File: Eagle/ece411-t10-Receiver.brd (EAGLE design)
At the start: 9.3 x 17.3 mm, 10 parts, among them X1 22-23-2021, X2 22-23-2021

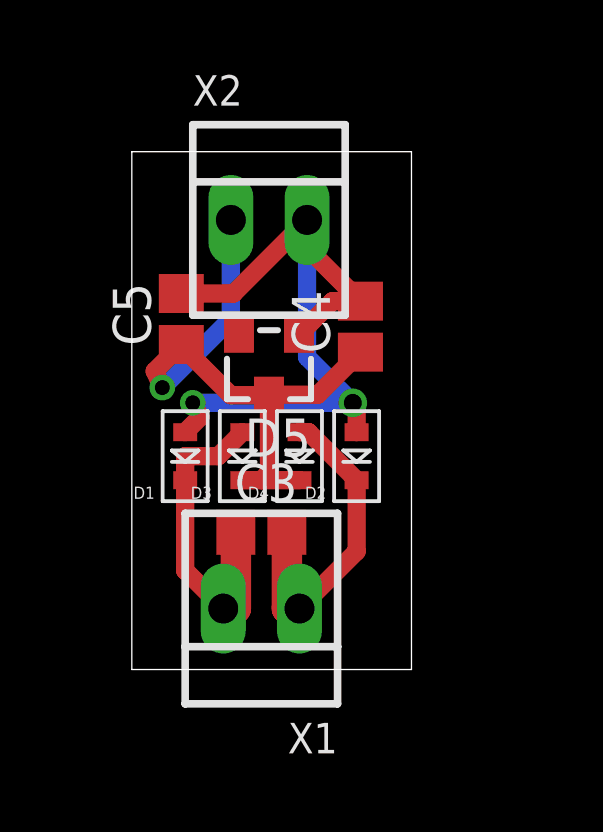
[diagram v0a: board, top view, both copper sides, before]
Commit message: Boards + schematics rev2
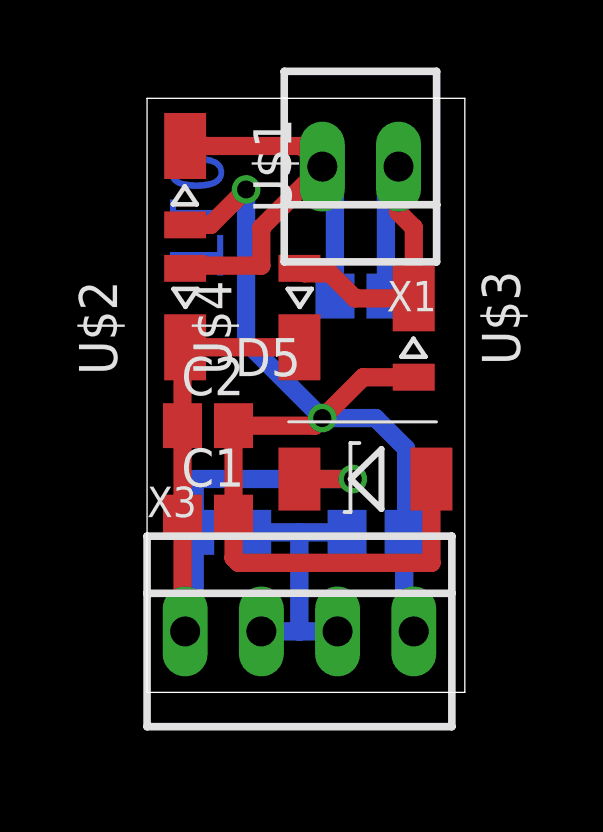
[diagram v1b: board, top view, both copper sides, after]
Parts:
- removed C4, C5: (no value), adafruit:C0805
- removed D1, D2, D3, D4: DFLS230LQ-7, adafruit:SOD-523
- removed X2: 22-23-2021, con-molex:22-23-2021
- added C1: 100n+, adafruit:C0805
- added C2: 100n, adafruit:C0805
- added R1: 75k, resistor:R0805
- added R2: 51k, resistor:R0805
- added U$1, U$2, U$3, U$4: DFLS230LQ-SCHOTTKY, _VMS:PWRDI123
- added X3: USB, con-molex:22-23-2041
- C3: value (none) -> NP
- D5: value 5.1V -> DZ2405100LCT-ZENER; device diode:TO236 -> _VMS:ZENER_PWR_PKG
- moved X1 15.1 mm to (7.11, 17.3)
- moved C3 8.54 mm to (7.11, 13.0), flipped to the bottom, turned to 180 degrees
- moved D5 3.94 mm to (5.08, 6.86), turned to 0 degrees
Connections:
- removed net N$3: C4.2, C5.2, D1.A, D2.A, D5.A, X2.2
- new net N$5: R1.1, R2.2, X3.2, X3.3
- new net N$8: C1.2, C2.2, D5.A, R2.1, U$1.A, U$3.A, X3.4
- net N$1: now also U$1.C, U$2.A; no longer D1.K, D3.A
- net N$2: now also U$3.C, U$4.A; no longer D2.K, D4.A
- net N$4: now also C1.1, C2.1, R1.2, U$2.C, U$4.C, X3.1; no longer C4.1, C5.1, D3.K, D4.K, X2.1
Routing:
- net N$8: track 0.00 -> 41.2 mm, vias 0 -> 2
- net N$3: track 25.5 -> 0.00 mm, vias 2 -> 0
- net N$5: track 0.00 -> 9.02 mm
- net N$1: track 10.8 -> 16.1 mm
- net N$4: track 20.5 -> 25.7 mm
- net N$2: track 10.6 -> 13.3 mm
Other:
- board size 9.3 x 17.3 mm -> 10.6 x 19.8 mm
- board text added: "T10"
